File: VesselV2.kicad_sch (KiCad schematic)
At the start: 208 parts, among them U1 ATmega32U4-A

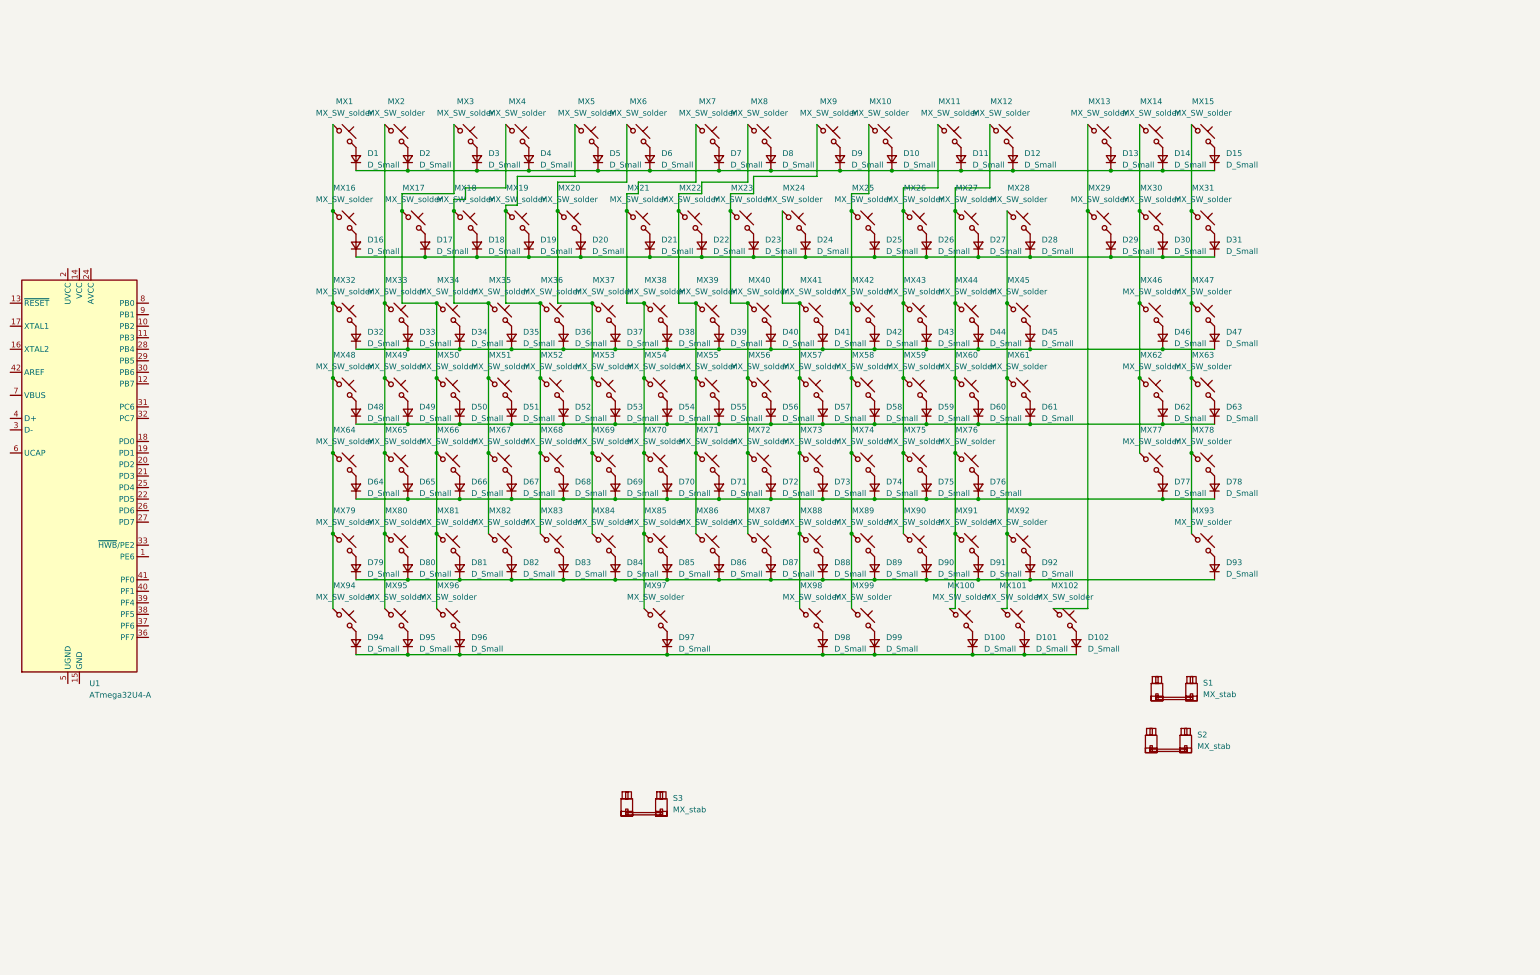
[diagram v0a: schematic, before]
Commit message: Footprint Assignment
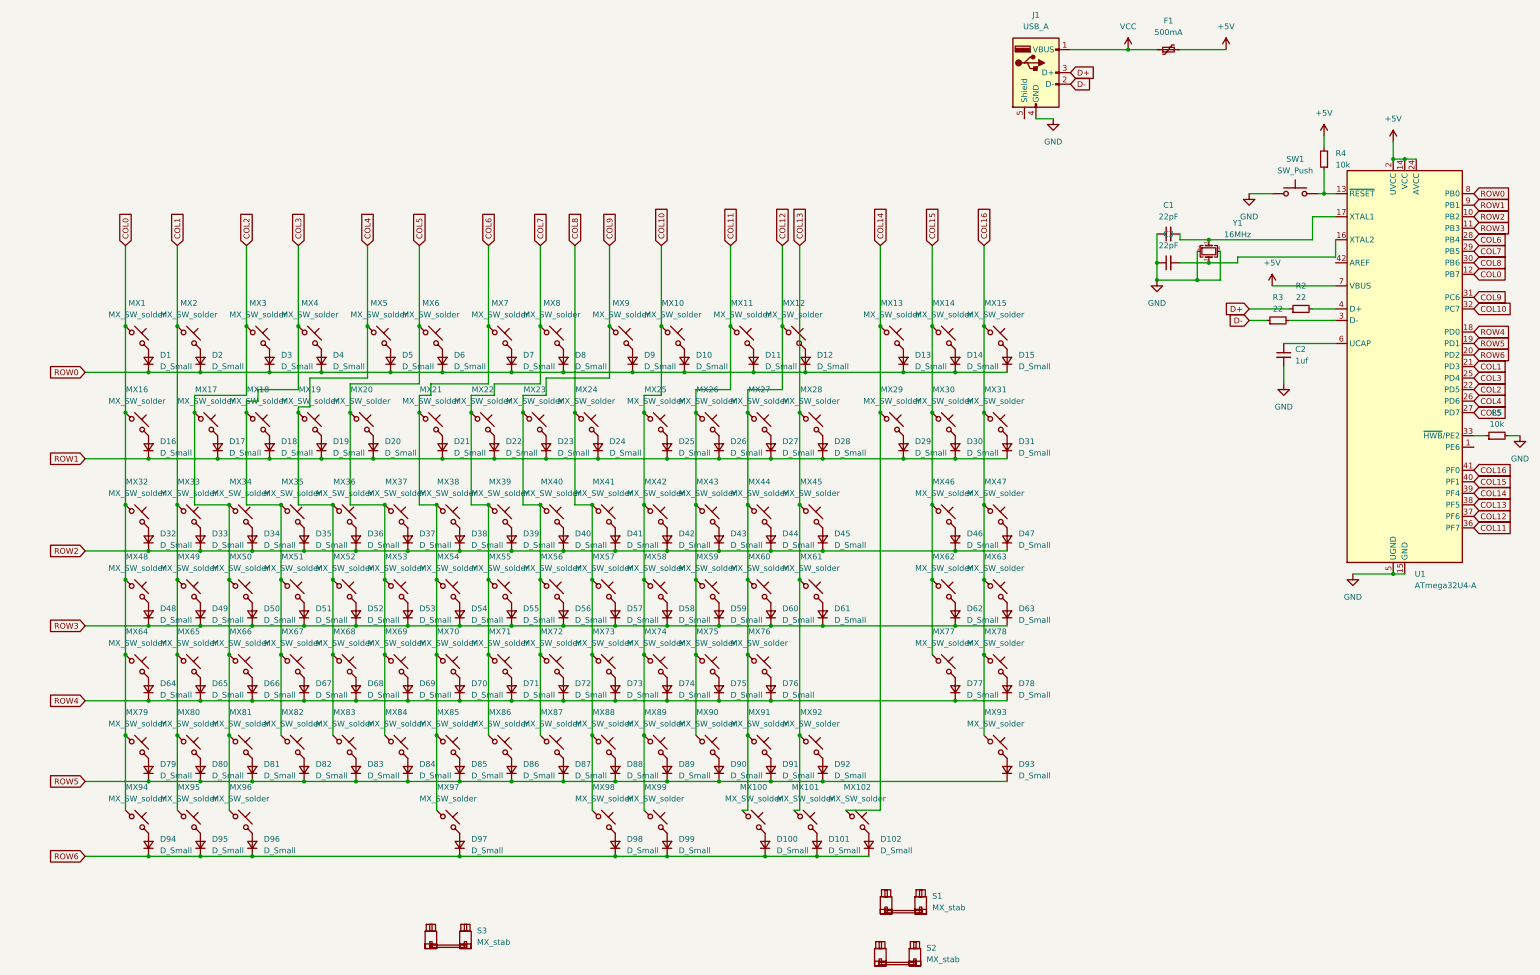
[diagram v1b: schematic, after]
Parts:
- added C1, C3: 22pF, Capacitor_SMD:C_0805_2012Metric_Pad1.18x1.45mm_HandSolder, symbol Device:C_Small
- added C2: 1uf, Capacitor_SMD:C_0805_2012Metric_Pad1.18x1.45mm_HandSolder, symbol Device:C_Small
- added F1: 500mA, Fuse:Fuse_1206_3216Metric_Pad1.42x1.75mm_HandSolder, symbol Device:Polyfuse_Small
- added J1: USB_A, Connector_USB:USB_A_Molex_67643_Horizontal, symbol Connector:USB_A
- added R2, R3: 22, Resistor_SMD:R_0805_2012Metric_Pad1.20x1.40mm_HandSolder, symbol Device:R_Small
- added R4, R5: 10k, Resistor_SMD:R_0805_2012Metric_Pad1.20x1.40mm_HandSolder, symbol Device:R_Small
- added SW1: SW_Push, symbol Switch:SW_Push
- added Y1: 16MHz, Crystal:Crystal_SMD_3225-4Pin_3.2x2.5mm_HandSoldering, symbol Device:Crystal_GND24_Small
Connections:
- net ROW6: now reaches D100.1 (K), D101.1 (K), D102.1 (K), D94.1 (K), D95.1 (K), D96.1 (K), D97.1 (K), D98.1 (K), D99.1 (K)
- net ROW6: now also U1.20 (PD2)
- net ROW2: now reaches U1.10 (PB2)
- net ROW2: now also D32.1 (K), D33.1 (K), D34.1 (K), D35.1 (K), D36.1 (K), D37.1 (K), D38.1 (K), D39.1 (K), D40.1 (K), D41.1 (K), D42.1 (K), D43.1 (K), D44.1 (K), D45.1 (K), D46.1 (K), D47.1 (K)
- net ROW3: now reaches U1.11 (PB3)
- net ROW3: now also D48.1 (K), D49.1 (K), D50.1 (K), D51.1 (K), D52.1 (K), D53.1 (K), D54.1 (K), D55.1 (K), D56.1 (K), D57.1 (K), D58.1 (K), D59.1 (K), D60.1 (K), D61.1 (K), D62.1 (K), D63.1 (K)
- net COL0: now reaches U1.12 (PB7)
- net COL0: now also MX1.1, MX16.1, MX32.1, MX48.1, MX64.1, MX79.1, MX94.1
- net at U1.13 (~{RESET}): now also R4.1, SW1.2
- net +5V: now reaches U1.14 (VCC), U1.34 (VCC)
- net +5V: now also U1.2 (UVCC), U1.24 (AVCC), U1.44 (AVCC), U1.7 (VBUS), F1.2, R4.2
- net GND: now reaches U1.15 (GND), U1.23 (GND), U1.35 (GND), U1.43 (GND)
- net GND: now also U1.5 (UGND), C1.1, C2.2, C3.1, J1.4 (GND), R5.2, SW1.1, Y1.2, Y1.4
- net at U1.16 (XTAL2): now also C3.2, Y1.3
- net at U1.17 (XTAL1): now also C1.2, Y1.1
- net ROW4: now reaches U1.18 (PD0)
- net ROW4: now also D64.1 (K), D65.1 (K), D66.1 (K), D67.1 (K), D68.1 (K), D69.1 (K), D70.1 (K), D71.1 (K), D72.1 (K), D73.1 (K), D74.1 (K), D75.1 (K), D76.1 (K), D77.1 (K), D78.1 (K)
- net ROW5: now reaches U1.19 (PD1)
- net ROW5: now also D79.1 (K), D80.1 (K), D81.1 (K), D82.1 (K), D83.1 (K), D84.1 (K), D85.1 (K), D86.1 (K), D87.1 (K), D88.1 (K), D89.1 (K), D90.1 (K), D91.1 (K), D92.1 (K), D93.1 (K)
- net COL1: now reaches U1.21 (PD3)
- net COL1: now also MX2.1, MX33.1, MX49.1, MX65.1, MX80.1, MX95.1
- net COL2: now reaches U1.22 (PD5)
- net COL2: now also MX17.1, MX3.1, MX34.1, MX50.1, MX66.1, MX81.1, MX96.1
- net COL3: now reaches U1.25 (PD4)
- net COL3: now also MX18.1, MX35.1, MX4.1, MX51.1, MX67.1, MX82.1
- net COL4: now reaches U1.26 (PD6)
- net COL4: now also MX19.1, MX36.1, MX5.1, MX52.1, MX68.1, MX83.1
- net COL5: now reaches U1.27 (PD7)
- net COL5: now also MX20.1, MX37.1, MX53.1, MX6.1, MX69.1, MX84.1
- net COL6: now reaches U1.28 (PB4)
- net COL6: now also MX21.1, MX38.1, MX54.1, MX7.1, MX70.1, MX85.1, MX97.1
- net COL7: now reaches U1.29 (PB5)
- net COL7: now also MX22.1, MX39.1, MX55.1, MX71.1, MX8.1, MX86.1
- net at U1.3 (D-): now also R3.2
- net COL8: now reaches U1.30 (PB6)
- net COL8: now also MX24.1, MX41.1, MX57.1, MX73.1, MX88.1, MX98.1
- net COL9: now reaches U1.31 (PC6)
- net COL9: now also MX23.1, MX40.1, MX56.1, MX72.1, MX87.1, MX9.1
- net COL10: now reaches U1.32 (PC7)
- net COL10: now also MX10.1, MX25.1, MX42.1, MX58.1, MX74.1, MX89.1, MX99.1
- net at U1.33 (~{HWB}/PE2): now also R5.1
- net COL11: now reaches U1.36 (PF7)
- net COL11: now also MX11.1, MX26.1, MX43.1, MX59.1, MX75.1, MX90.1
- net COL12: now reaches U1.37 (PF6)
- net COL12: now also MX100.1, MX12.1, MX27.1, MX44.1, MX60.1, MX76.1, MX91.1
- net COL13: now reaches U1.38 (PF5)
- net COL13: now also MX101.1, MX28.1, MX45.1, MX61.1, MX92.1
- net COL14: now reaches U1.39 (PF4)
- net COL14: now also MX102.1, MX13.1, MX29.1
- net at U1.4 (D+): now also R2.2
- net COL15: now reaches U1.40 (PF1)
- net COL15: now also MX14.1, MX30.1, MX46.1, MX62.1, MX77.1
- net COL16: now reaches U1.41 (PF0)
- net COL16: now also MX15.1, MX31.1, MX47.1, MX63.1, MX78.1, MX93.1
- net at U1.6 (UCAP): now also C2.1
- net ROW0: now reaches U1.8 (PB0)
- net ROW0: now also D1.1 (K), D10.1 (K), D11.1 (K), D12.1 (K), D13.1 (K), D14.1 (K), D15.1 (K), D2.1 (K), D3.1 (K), D4.1 (K), D5.1 (K), D6.1 (K), D7.1 (K), D8.1 (K), D9.1 (K)
- net ROW1: now reaches U1.9 (PB1)
- net ROW1: now also D16.1 (K), D17.1 (K), D18.1 (K), D19.1 (K), D20.1 (K), D21.1 (K), D22.1 (K), D23.1 (K), D24.1 (K), D25.1 (K), D26.1 (K), D27.1 (K), D28.1 (K), D29.1 (K), D30.1 (K), D31.1 (K)
- new net D+: J1.3 (D+), R2.1
- new net D-: J1.2 (D-), R3.1
- new net VCC: F1.1, J1.1 (VBUS)
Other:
- moved on the sheet: D1, D10, D100, D101, D102, D11, D12, D13, D14, D15, D16, D17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
